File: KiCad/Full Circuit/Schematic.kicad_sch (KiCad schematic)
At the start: 44 parts, among them U1 LMH6609MF, U2 LMH6609MF, U3 LMH6609MF, U4 LMH6609MF, U5 LMH6609MF, U6 LMH6609MF

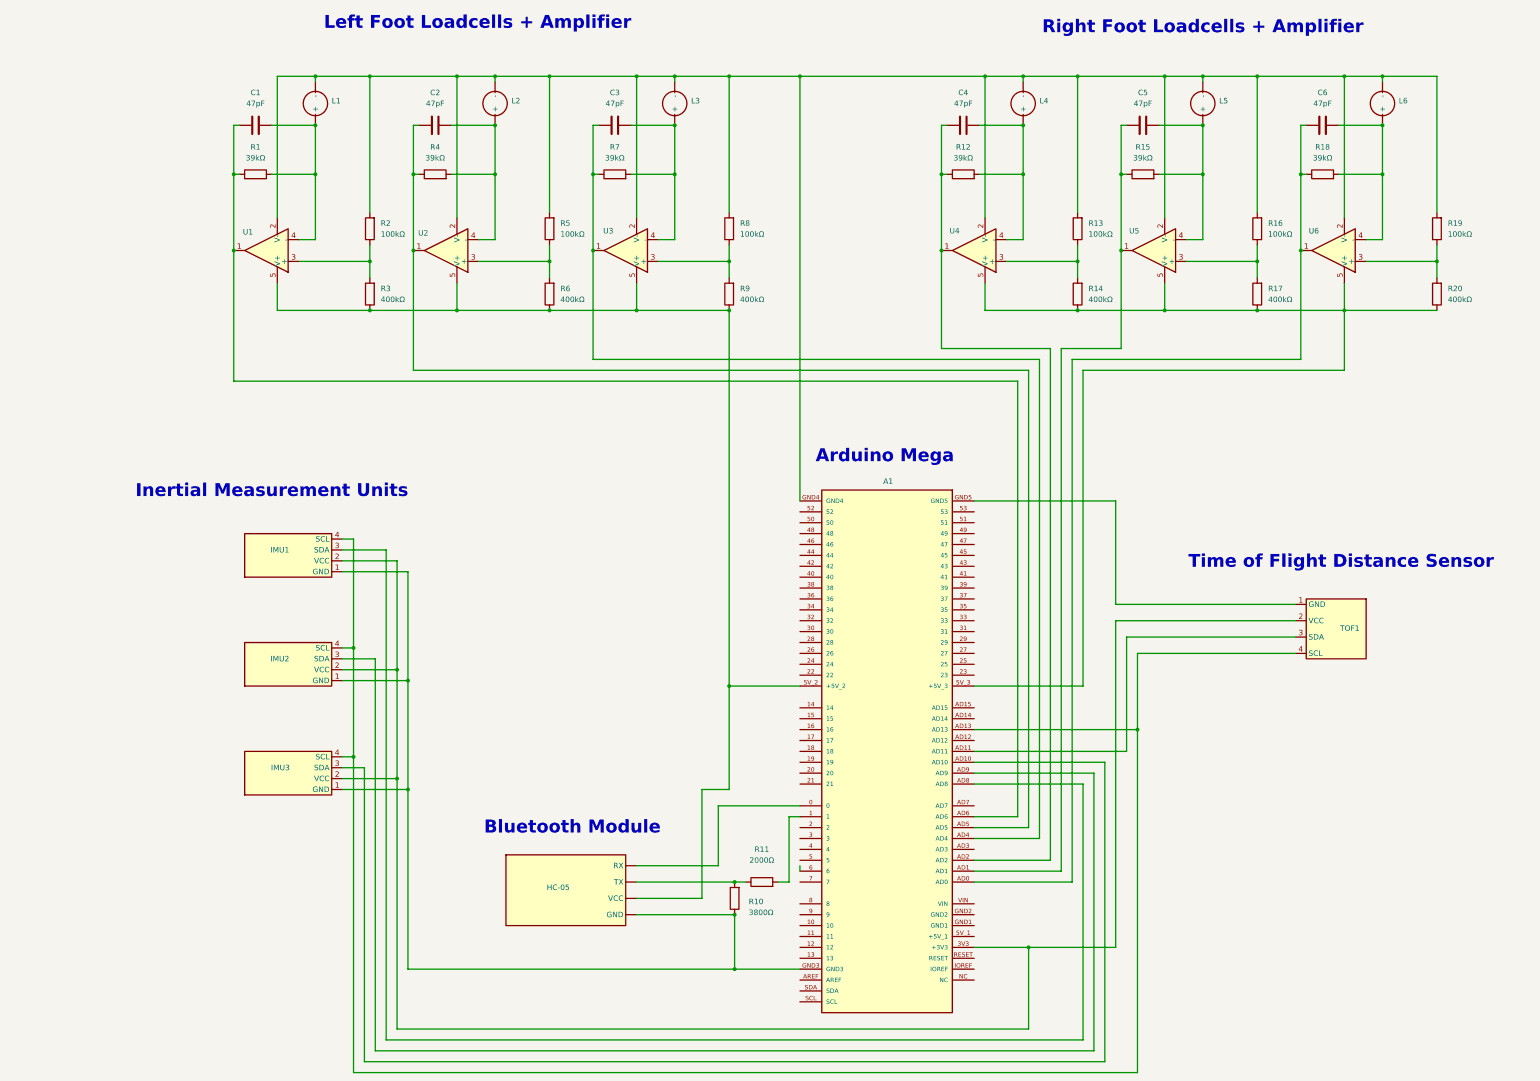
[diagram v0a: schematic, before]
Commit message: uppdate
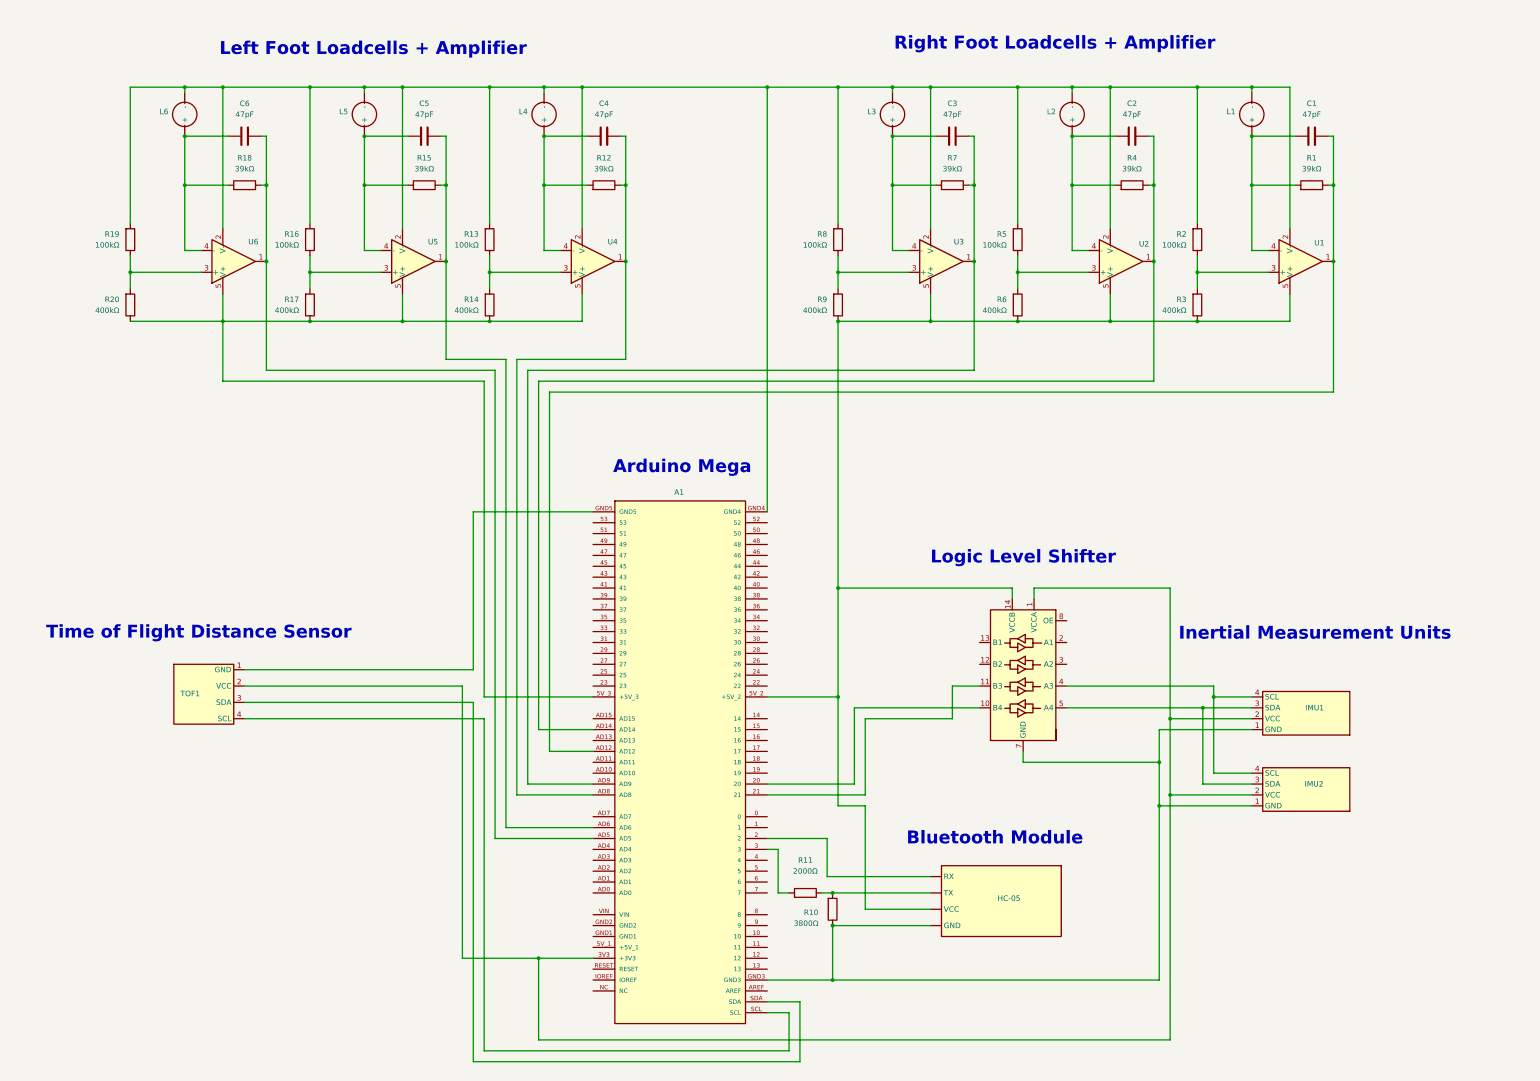
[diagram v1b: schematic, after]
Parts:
- removed IMU1: ~, symbol ProjectSymbols:Grove IMU 9DOF
- added U7: TXB0104PW, Package_SO:TSSOP-14_4.4x5mm_P0.65mm, symbol Logic_LevelTranslator:TXB0104PW
- renumbered IMU2 to IMU1, IMU3 to IMU2
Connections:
- net at C6.1, R18.1, U6.1: now also A1.AD5; no longer A1.AD0
- net at C2.2, R4.1, U2.1: now also A1.AD14; no longer A1.AD5
- net at A1.5V_2 (+5V_2), HC-05. (GND), R3.1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: now also U7.14 (VCCB)
- net at C4.2, R12.1, U4.1: now also A1.AD8; no longer A1.AD2
- net at C3.1, R7.1, U3.1: now also A1.AD9; no longer A1.AD4
- net at C5.2, R15.1, U5.1: now also A1.AD6; no longer A1.AD1
- net at A1.GND3, HC-05. (GND), IMU1.1 (GND)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: now also U7.7 (GND)
- net at A1.3V3 (+3V3), IMU1.2 (VCC), IMU2.2 (VCC)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: now also U7.1 (VCCA)
- net at IMU1.3 (SDA): now also IMU2.3 (SDA), U7.5 (A4); no longer A1.AD9
- net at IMU1.4 (SCL), IMU2.4 (SCL): now also U7.4 (A3); no longer A1.AD13, TOF1.4 (SCL)
- net at R11.2: now also A1.3; no longer A1.1
- net at A1.0: no longer HC-05. (GND)
- net at A1.2: now also HC-05. (GND)
- net at A1.20: now also U7.10 (B4)
- net at A1.21: now also U7.11 (B3)
- net at A1.AD10: no longer IMU2.3 (SDA)
- net at A1.AD11: no longer TOF1.3 (SDA)
- net at A1.AD12: now also C1.2, R1.1, U1.1
- net at A1.SCL: now also TOF1.4 (SCL)
- net at A1.SDA: now also TOF1.3 (SDA)
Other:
- note added: "Logic Level Shifter"
- moved on the sheet: A1, C1, C2, C3, C4, C5, C6, HC-05, IMU1, IMU2, L1, L2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
